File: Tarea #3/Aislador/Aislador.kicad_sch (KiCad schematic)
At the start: 31 parts, among them IC1 MIE1W0505BGLVH-3R-P, U1 ADUM3160BRWZ

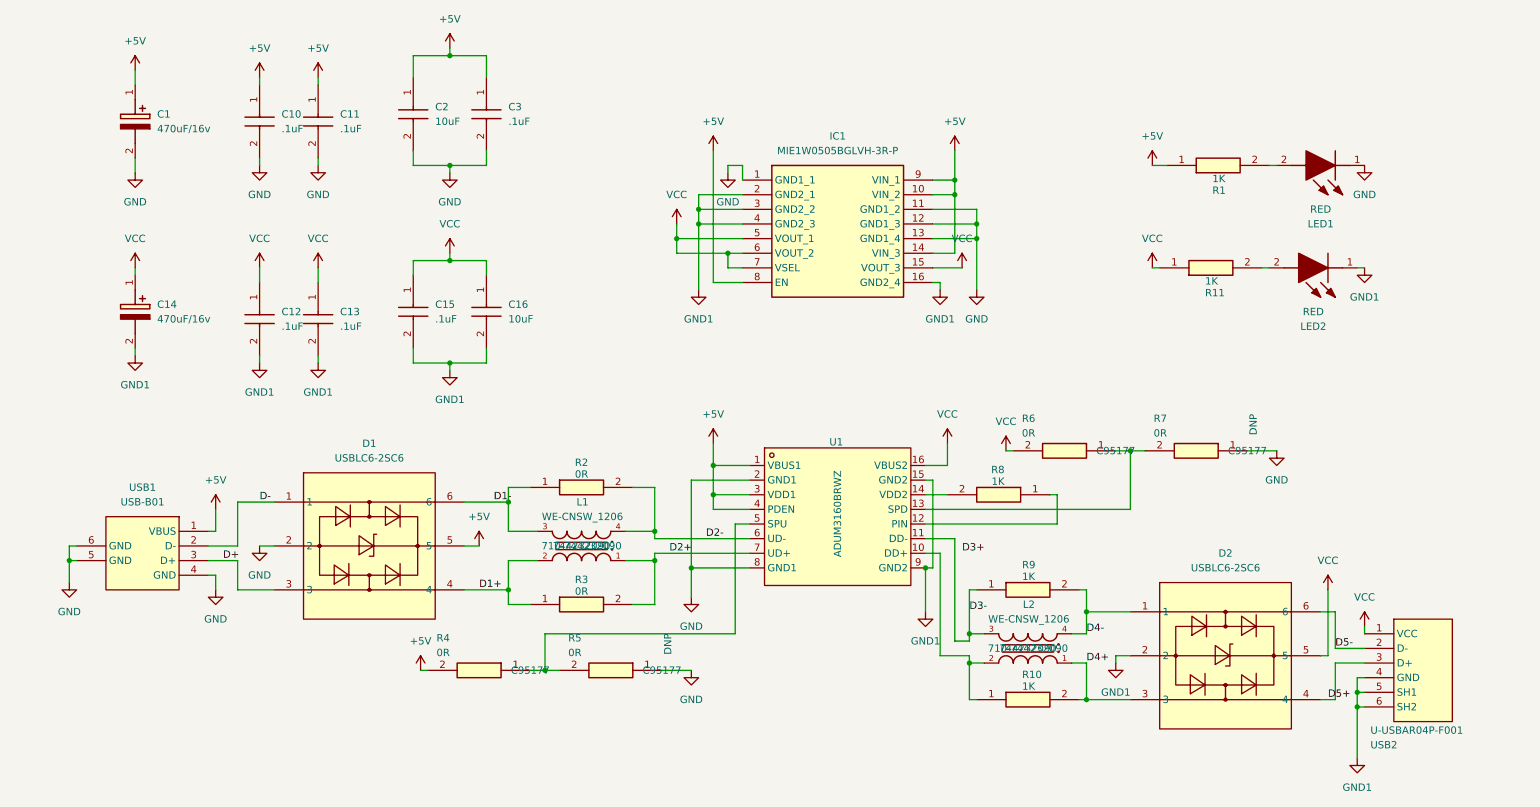
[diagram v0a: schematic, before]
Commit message: Aislador
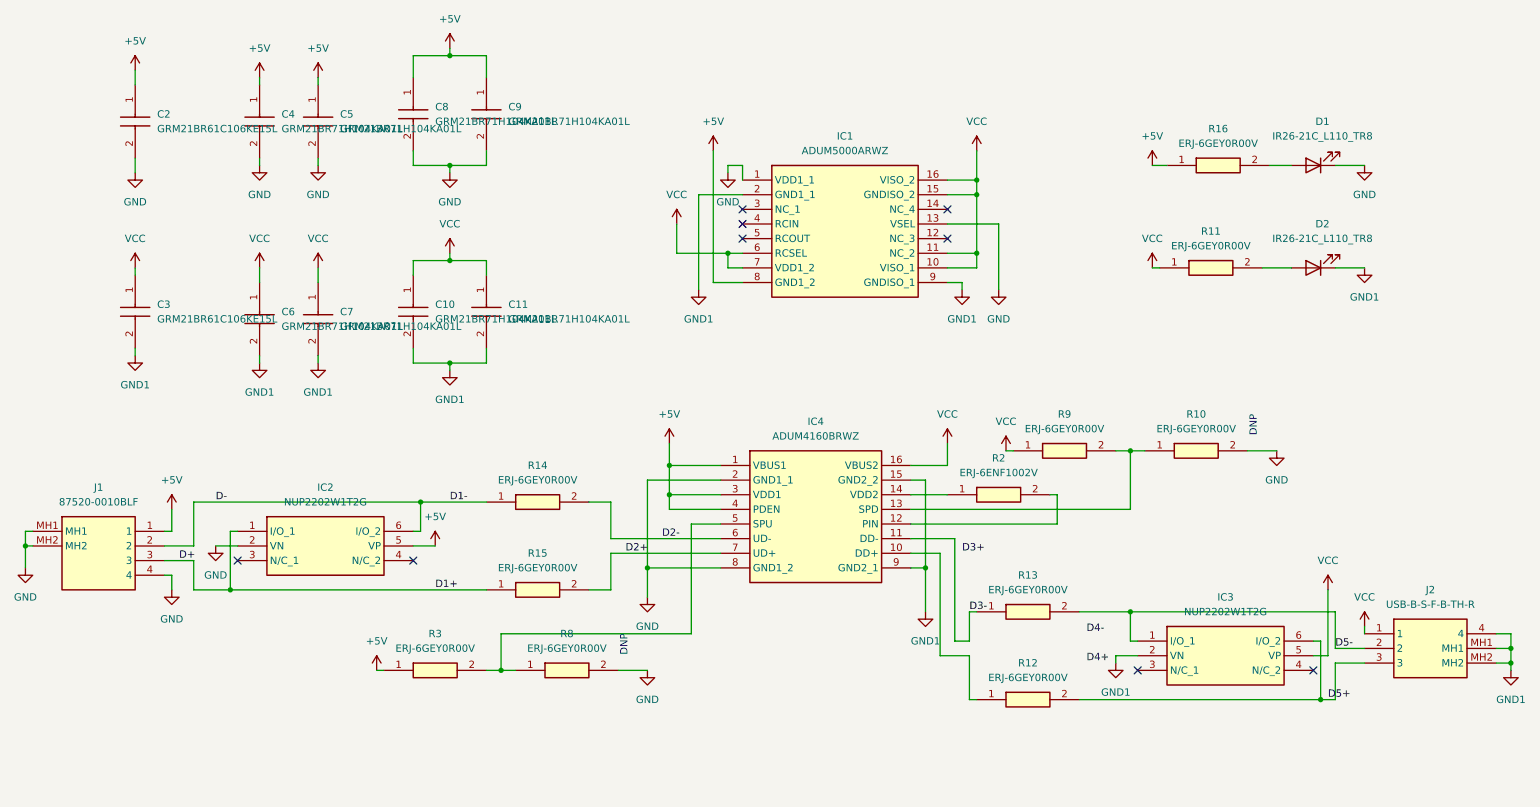
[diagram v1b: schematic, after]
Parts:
- removed C1, C14: 470uF/16v, Samacsys:EEE1AA220WR, symbol Samacsys:EEE-FN1C470UR
- removed C10, C11, C12, C13, C15, C3: .1uF, Samacsys:CAPC1608X90N, symbol Samacsys:0603YC104J4T2A
- removed C16, C2: 10uF, Samacsys:CAPC1608X102N, symbol Samacsys:0603YD106KAT2A
- removed D1, D2: USBLC6-2SC6, EasyEDA:SOT-23-6_L2.9-W1.6-P0.95-LS2.8-BL, symbol EasyEDA:USBLC6-2SC6
- removed IC1: MIE1W0505BGLVH-3R-P, Samacsys:MIE1W0505BGLVH3RP, symbol Samacsys:MIE1W0505BGLVH-3R-P
- removed L1, L2: WE-CNSW_1206, Snapeda:WE-CNSW_1206_WE-CNSW_1206, symbol Snapeda:WE-CNSW_1206
- removed LED1, LED2: RED, Samacsys:KSEELP4122P1R258A8J8020R18, symbol Samacsys:KS_EELP41.22-P1R2-58-A8J8-020-R18
- removed R1, R10, R11, R8, R9: 1K, Samacsys:RESC1608X55N, symbol Samacsys:RT0603FRE071KL
- removed R2, R3, R4, R5, R6, R7: 0R, Samacsys:RESC1608X55N, symbol Samacsys:RC0603FR-070RL
- removed U1: ADUM3160BRWZ, EasyEDA:WSOIC-16_L10.3-W7.5-P1.27-LS10.3-BL, symbol EasyEDA:ADUM3160BRWZ
- removed USB1: USB-B01, EasyEDA:USB-B-TH_USB-B01, symbol EasyEDA:USB-B01
- removed USB2: U-USBAR04P-F001, EasyEDA:USB-A-TH_USB-302-T, symbol EasyEDA:U-USBAR04P-F001
- added C10, C11, C4, C5, C6, C7, C8, C9: GRM21BR71H104KA01L, SamacSys_Parts:CAPC2012X145N, symbol SamacSys_Parts:GRM21BR71H104KA01L
- added C2, C3: GRM21BR61C106KE15L, SamacSys_Parts:CAPC2012X145N, symbol SamacSys_Parts:GRM21BR61C106KE15L
- added D1, D2: IR26-21C_L110_TR8, LED_SMD:LED_1206_3216Metric, symbol LED:IR26-21C_L110_TR8
- added IC1: ADUM5000ARWZ, SamacSys_Parts:SOIC127P1032X265-16N, symbol SamacSys_Parts:ADUM5000ARWZ
- added IC2, IC3: NUP2202W1T2G, SamacSys_Parts:SOT65P210X110-6N, symbol SamacSys_Parts:NUP2202W1T2G
- added IC4: ADUM4160BRWZ, SOIC127P1032X265-16N, symbol SamacSys_Parts:ADUM4160BRWZ
- added J1: 87520-0010BLF, SamacSys_Parts:875200010BLF, symbol SamacSys_Parts:87520-0010BLF
- added J2: USB-B-S-F-B-TH-R, SamacSys_Parts:USBBSFBTHR, symbol SamacSys_Parts:USB-B-S-F-B-TH-R
- added R10, R11, R12, R13, R14, R15, R16, R3, R8, R9: ERJ-6GEY0R00V, SamacSys_Parts:RESC2012X70N, symbol SamacSys_Parts:ERJ-6GEY0R00V
- added R2: ERJ-6ENF1002V, SamacSys_Parts:ERJ6ENF1000V, symbol SamacSys_Parts:ERJ-6ENF1002V
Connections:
- net +5V: now also C2.1, C4.1, C5.1, C8.1, C9.1, IC1.8 (GND1_2), IC2.5 (VP), IC4.1 (VBUS1), IC4.3 (VDD1), IC4.4 (PDEN), J1.1, R16.1, R3.1
- net D+: now also IC2.1 (I/O_1), J1.3, R15.1
- net D-: now also IC2.6 (I/O_2), J1.2, R14.1
- net D2+: now also IC4.7 (UD+), R15.2
- net D2-: now also IC4.6 (UD-), R14.2
- net D3-: now also IC4.11 (DD-), R13.1
- net D5+: now also IC3.6 (I/O_2), J2.3, R12.2
- net D5-: now also IC3.1 (I/O_1), J2.2, R13.2
- net GND: now also C2.2, C4.2, C5.2, C8.2, C9.2, D1.1 (K), IC1.1 (VDD1_1), IC1.13 (VSEL), IC2.2 (VN), IC4.2 (GND1_1), IC4.8 (GND1_2), J1.4, J1.MH1, J1.MH2, R10.2, R8.2
- net GND1: now also C10.2, C11.2, C3.2, C6.2, C7.2, D2.1 (K), IC1.2 (GND1_1), IC1.9 (GNDISO_1), IC3.2 (VN), IC4.15 (GND2_2), IC4.9 (GND2_1), J2.4, J2.MH1, J2.MH2
- net VCC: now also C10.1, C11.1, C3.1, C6.1, C7.1, IC1.10 (VISO_1), IC1.11 (NC_2), IC1.15 (GNDISO_2), IC1.16 (VISO_2), IC1.6 (RCSEL), IC1.7 (VDD1_2), IC3.5 (VP), IC4.16 (VBUS2), J2.1, R11.1, R9.1
- new net: D2.2 (A), R11.2
- new net: D1.2 (A), R16.2
- new net: IC4.5 (SPU), R3.2, R8.1
- new net: IC4.13 (SPD), R10.1, R9.2
- new net: IC4.10 (DD+), R12.1
- new net: IC4.12 (PIN), R2.2
- new net: IC4.14 (VDD2), R2.1
- no-connect marks 0 -> 9
